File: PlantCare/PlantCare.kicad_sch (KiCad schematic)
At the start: 21 parts, among them J1 USB4105-GF-A, U1 AMS1117-3.3, U2 ESP32-S3-WROOM-1-N16R2

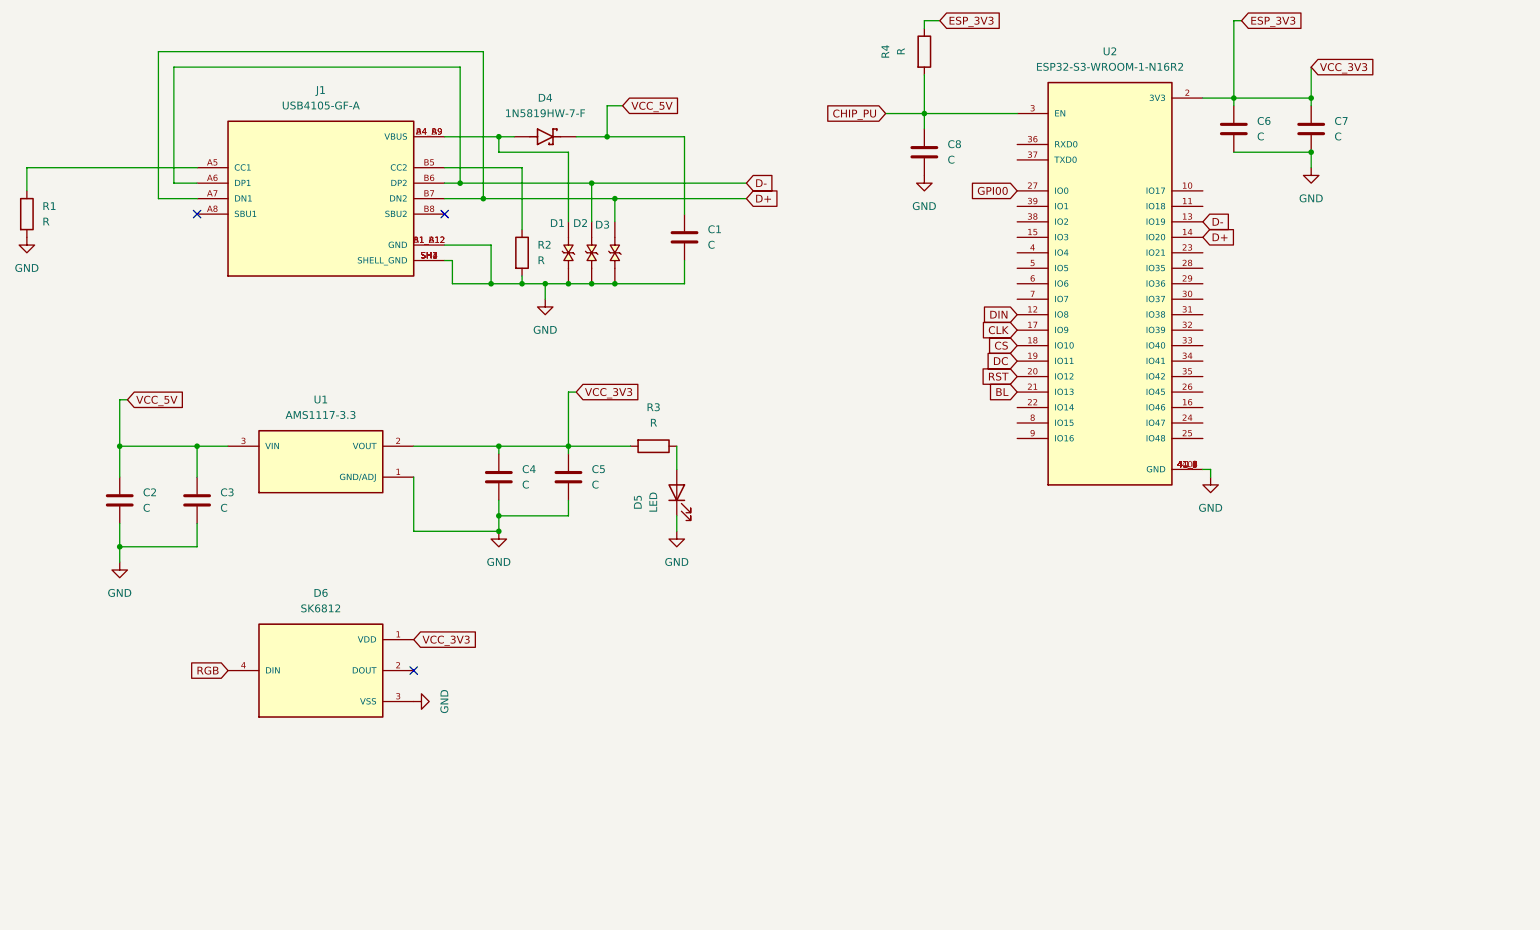
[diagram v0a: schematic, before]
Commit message: Add complete schemes
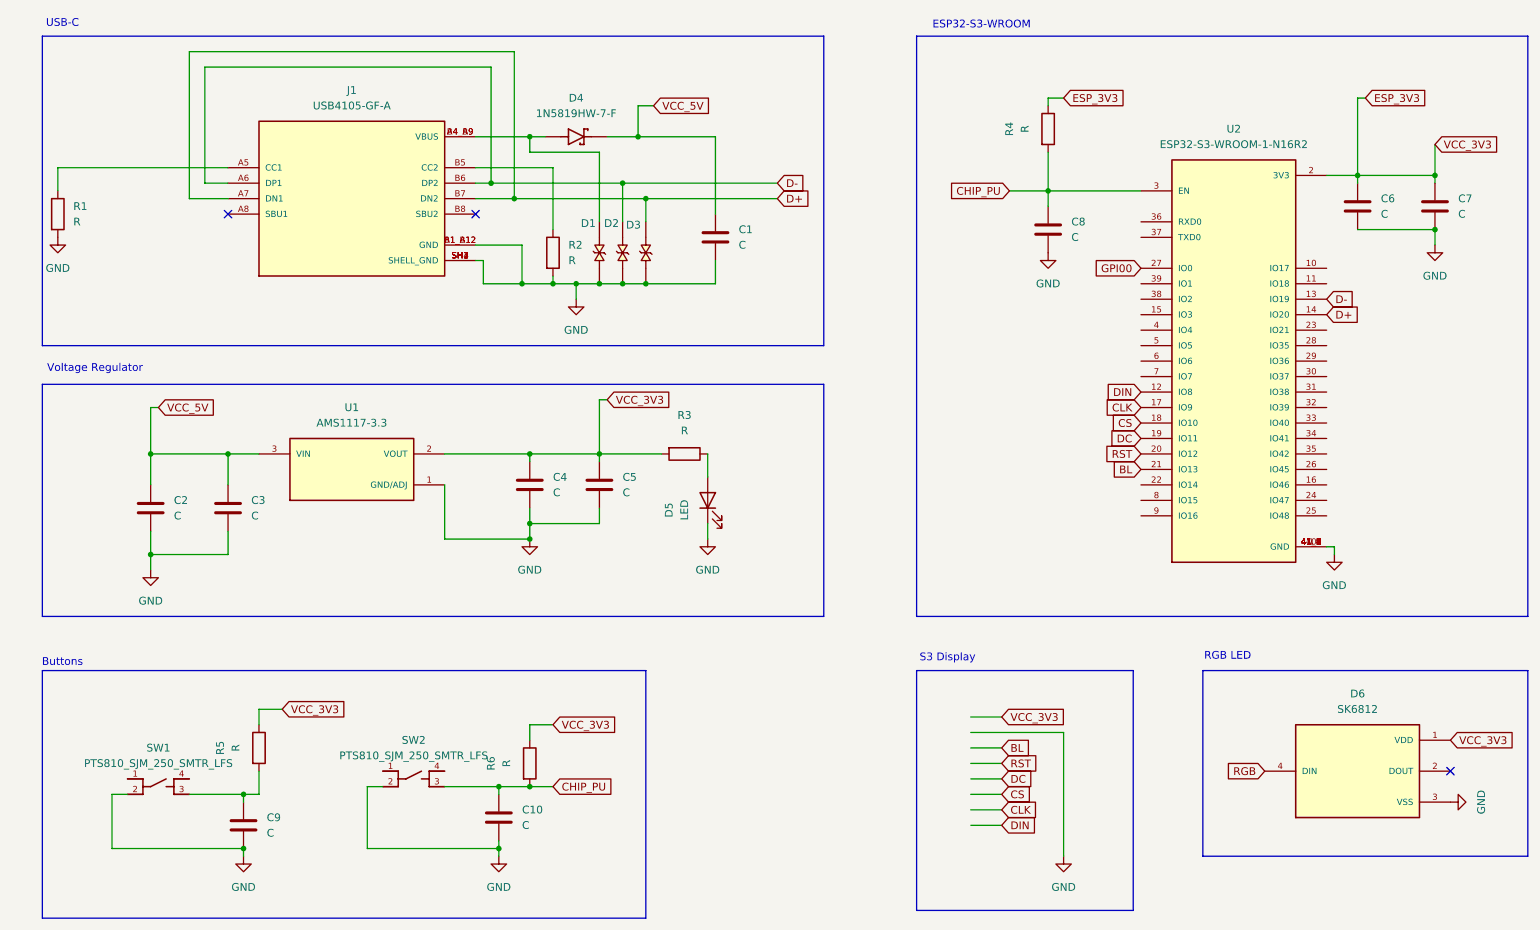
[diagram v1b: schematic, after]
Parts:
- added C10, C9: C, symbol Device:C
- added R5, R6: R, symbol Device:R
- added SW1, SW2: PTS810_SJM_250_SMTR_LFS, SW_PTS810_SJM_250_SMTR_LFS, symbol PTS810_SJM_250_SMTR_LFS:PTS810_SJM_250_SMTR_LFS
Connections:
- net CHIP_PU: now also C10.1, R6.2, SW2.3
- net ESP_3V3: now also R5.1, R6.1
- net GND: now also C10.2, C9.2, SW1.2, SW2.2
- new net: C9.1, R5.2, SW1.3
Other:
- note added: "Buttons"
- note added: "ESP32-S3-WROOM"
- note added: "RGB LED"
- note added: "S3 Display"
- note added: "USB-C"
- note added: "Voltage Regulator"
- title: (none) -> PLANTCARE MOISTURE MODULE SCHEME
- moved on the sheet: C1, C2, C3, C4, C5, C6, C7, C8, D1, D2, D3, D4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

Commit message: Link footprints
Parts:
- C1, C10, C2, C3, C4, C5, C6, C7, C8, C9: footprint (none) -> Capacitor_Tantalum_SMD:CP_EIA-1608-08_AVX-J
- D1, D2, D3: footprint TVS_LESD5D5.0CT1G -> LESD5D5.0CT1G-footprint:TVS_LESD5D5.0CT1G
- D4: footprint SOD3715X145N -> 1N5819HW-7-F-footprint:SOD3715X145N
- D5: footprint (none) -> Diode_SMD:D_0805_2012Metric
- D6: footprint LED_SK6812 -> SK6812-footprint:LED_SK6812
- J1: footprint GCT_USB4105-GF-A -> USB4105-GF-A-footprint:GCT_USB4105-GF-A
- R1, R2, R3, R4, R5, R6: footprint (none) -> Resistor_SMD:R_0201_0603Metric
- SW1, SW2: footprint SW_PTS810_SJM_250_SMTR_LFS -> PTS810_SJM_250_SMTR_LFS-footprint:SW_PTS810_SJM_250_SMTR_LFS
- U1: footprint SOT229P700X180-4N -> AMS1117-3.3-footprint:SOT229P700X180-4N
- U2: footprint XCVR_ESP32-S3-WROOM-1-N16R2 -> ESP32-S3-WROOM-1-N16R2-footprint:XCVR_ESP32-S3-WROOM-1-N16R2
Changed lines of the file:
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@@
 			)
 		)
-		(property "Footprint" ""
+		(property "Footprint" "Resistor_SMD:R_0201_0603Metric"
 			(at 21.082 48.26 90)
 			(effects
@@
 			)
 		)
-		(property "Footprint" ""
+		(property "Footprint" "Resistor_SMD:R_0201_0603Metric"
 			(at 125.73 85.852 90)
 			(effects
@@
 			)
 		)
-		(property "Footprint" ""
+		(property "Footprint" "Capacitor_Tantalum_SMD:CP_EIA-1608-08_AVX-J"
 			(at 51.7652 100.33 0)
 			(effects
@@
 			)
 		)
-		(property "Footprint" ""
+		(property "Footprint" "Resistor_SMD:R_0201_0603Metric"
 			(at 183.642 34.29 90)
 			(effects
@@
 			)
 		)
-		(property "Footprint" ""
+		(property "Footprint" "Capacitor_Tantalum_SMD:CP_EIA-1608-08_AVX-J"
 			(at 112.7252 96.52 0)
 			(effects
@@
 			)
 		)
-		(property "Footprint" "TVS_LESD5D5.0CT1G"
+		(property "Footprint" "LESD5D5.0CT1G-footprint:TVS_LESD5D5.0CT1G"
 			(at 115.57 54.61 0)
 			(effects
@@
 			)
 		)
-		(property "Footprint" "SW_PTS810_SJM_250_SMTR_LFS"
+		(property "Footprint" "PTS810_SJM_250_SMTR_LFS-footprint:SW_PTS810_SJM_250_SMTR_LFS"
 			(at 81.28 139.7 0)
 			(effects
@@
 			)
 		)
-		(property "Footprint" ""
+		(property "Footprint" "Capacitor_Tantalum_SMD:CP_EIA-1608-08_AVX-J"
 			(at 186.3852 54.61 0)
 			(effects
@@
 			)
 		)
-		(property "Footprint" ""
+		(property "Footprint" "Diode_SMD:D_0805_2012Metric"
 			(at 129.54 95.25 0)
 			(effects
@@
 			)
 		)
-		(property "Footprint" ""
+		(property "Footprint" "Capacitor_Tantalum_SMD:CP_EIA-1608-08_AVX-J"
 			(at 249.8852 50.8 0)
 			(effects
@@
 			)
 		)
-		(property "Footprint" "LED_SK6812"
+		(property "Footprint" "SK6812-footprint:LED_SK6812"
 			(at 236.22 139.7 0)
 			(effects
@@
 			)
 		)
-		(property "Footprint" "TVS_LESD5D5.0CT1G"
+		(property "Footprint" "LESD5D5.0CT1G-footprint:TVS_LESD5D5.0CT1G"
 			(at 111.76 54.61 0)
 			(effects
@@
 			)
 		)
-		(property "Footprint" ""
+		(property "Footprint" "Resistor_SMD:R_0201_0603Metric"
 			(at 98.552 138.43 90)
 			(effects
@@
 			)
 		)
-		(property "Footprint" ""
+		(property "Footprint" "Capacitor_Tantalum_SMD:CP_EIA-1608-08_AVX-J"
 			(at 54.3052 152.4 0)
 			(effects
@@
 			)
 		)
-		(property "Footprint" "SOD3715X145N"
+		(property "Footprint" "1N5819HW-7-F-footprint:SOD3715X145N"
 			(at 107.95 35.56 0)
 			(effects
@@
 			)
 		)
-		(property "Footprint" "SOT229P700X180-4N"
+		(property "Footprint" "AMS1117-3.3-footprint:SOT229P700X180-4N"
 			(at 71.12 90.17 0)
 			(effects
@@
 			)
 		)
-		(property "Footprint" ""
+		(property "Footprint" "Capacitor_Tantalum_SMD:CP_EIA-1608-08_AVX-J"
 			(at 131.7752 55.88 0)
 			(effects
@@
 			)
 		)
-		(property "Footprint" ""
+		(property "Footprint" "Capacitor_Tantalum_SMD:CP_EIA-1608-08_AVX-J"
 			(at 96.2152 151.13 0)
 			(effects
@@
 			)
 		)
-		(property "Footprint" ""
+		(property "Footprint" "Capacitor_Tantalum_SMD:CP_EIA-1608-08_AVX-J"
 			(at 237.1852 50.8 0)
 			(effects
@@
 			)
 		)
-		(property "Footprint" "GCT_USB4105-GF-A"
+		(property "Footprint" "USB4105-GF-A-footprint:GCT_USB4105-GF-A"
 			(at 71.12 45.72 0)
 			(effects
@@
 			)
 		)
-		(property "Footprint" ""
+		(property "Footprint" "Resistor_SMD:R_0201_0603Metric"
 			(at 54.102 135.89 90)
 			(effects
@@
 			)
 		)
-		(property "Footprint" "XCVR_ESP32-S3-WROOM-1-N16R2"
+		(property "Footprint" "ESP32-S3-WROOM-1-N16R2-footprint:XCVR_ESP32-S3-WROOM-1-N16R2"
 			(at 215.9 72.39 0)
 			(effects
@@
 			)
 		)
-		(property "Footprint" "SW_PTS810_SJM_250_SMTR_LFS"
+		(property "Footprint" "PTS810_SJM_250_SMTR_LFS-footprint:SW_PTS810_SJM_250_SMTR_LFS"
 			(at 39.37 140.97 0)
 			(effects
@@
 			)
 		)
-		(property "Footprint" ""
+		(property "Footprint" "Capacitor_Tantalum_SMD:CP_EIA-1608-08_AVX-J"
 			(at 101.2952 96.52 0)
 			(effects
@@
 			)
 		)
-		(property "Footprint" ""
+		(property "Footprint" "Capacitor_Tantalum_SMD:CP_EIA-1608-08_AVX-J"
 			(at 39.0652 100.33 0)
 			(effects
@@
 			)
 		)
-		(property "Footprint" ""
+		(property "Footprint" "Resistor_SMD:R_0201_0603Metric"
 			(at 102.362 54.61 90)
 			(effects
@@
 			)
 		)
-		(property "Footprint" "TVS_LESD5D5.0CT1G"
+		(property "Footprint" "LESD5D5.0CT1G-footprint:TVS_LESD5D5.0CT1G"
 			(at 119.38 54.61 0)
 			(effects

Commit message: Clean scheme
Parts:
- removed C1, C10, C2, C3, C4, C5, C6, C7, C8, C9: C, Capacitor_Tantalum_SMD:CP_EIA-1608-08_AVX-J, symbol Device:C
- removed D1, D2, D3: ~, LESD5D5.0CT1G-footprint:TVS_LESD5D5.0CT1G, symbol LESD5D5.0CT1G:LESD5D5.0CT1G
- removed D4: 1N5819HW-7-F, 1N5819HW-7-F-footprint:SOD3715X145N, symbol 1N5819HW-7-F:1N5819HW-7-F
- removed D5: LED, Diode_SMD:D_0805_2012Metric, symbol Device:LED
- removed D6: SK6812, SK6812-footprint:LED_SK6812, symbol SK6812:SK6812
- removed J1: USB4105-GF-A, USB4105-GF-A-footprint:GCT_USB4105-GF-A, symbol USB4105-GF-A:USB4105-GF-A
- removed R1, R2, R3, R4, R5, R6: R, Resistor_SMD:R_0201_0603Metric, symbol Device:R
- removed SW1, SW2: PTS810_SJM_250_SMTR_LFS, PTS810_SJM_250_SMTR_LFS-footprint:SW_PTS810_SJM_250_SMTR_LFS, symbol PTS810_SJM_250_SMTR_LFS:PTS810_SJM_250_SMTR_LFS
- removed U1: AMS1117-3.3, AMS1117-3.3-footprint:SOT229P700X180-4N, symbol AMS1117-3.3:AMS1117-3.3
- removed U2: ESP32-S3-WROOM-1-N16R2, ESP32-S3-WROOM-1-N16R2-footprint:XCVR_ESP32-S3-WROOM-1-N16R2, symbol ESP32-S3-WROOM-1-N16R2:ESP32-S3-WROOM-1-N16R2
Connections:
- no-connect marks 3 -> 0
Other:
- note removed: "Buttons"
- note removed: "ESP32-S3-WROOM"
- note removed: "RGB LED"
- note removed: "S3 Display"
- note removed: "USB-C"
- note removed: "Voltage Regulator"
